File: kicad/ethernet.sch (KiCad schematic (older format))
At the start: 32 parts, among them IC201 TPD4E001QDBV, J201 0821-1X1T-36-F, U201 DP83822

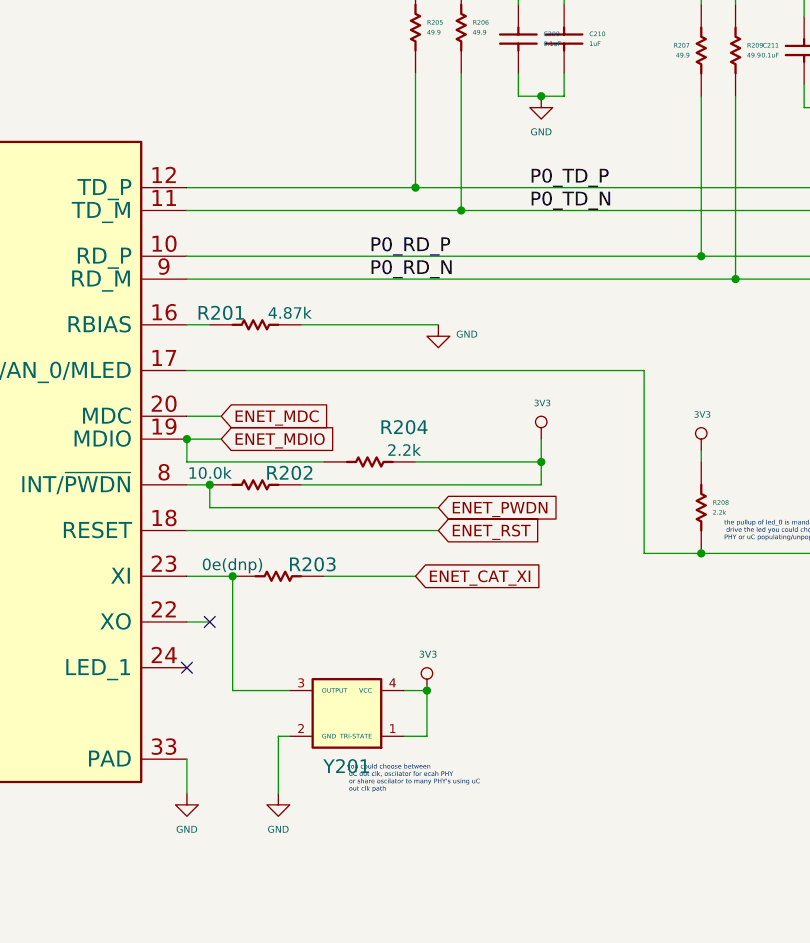
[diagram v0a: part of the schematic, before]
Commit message: keep placing
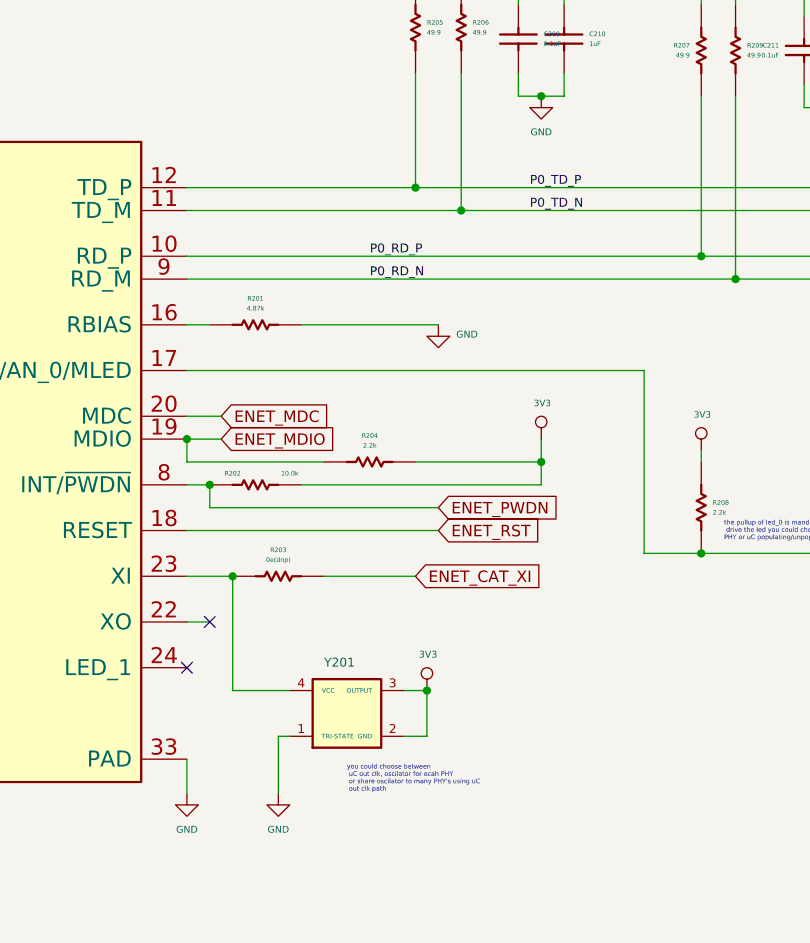
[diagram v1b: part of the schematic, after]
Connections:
- net 3V3: now also R204.2, Y201.2 (GND), Y201.3 (OUTPUT); no longer R204.1, Y201.1 (TRI-STATE), Y201.4 (VCC)
- net ENET_MDIO: now also R204.1; no longer R204.2
- net GND: now also Y201.1 (TRI-STATE); no longer Y201.2 (GND)
- net at R203.1, U201.23 (XI): now also Y201.4 (VCC); no longer Y201.3 (OUTPUT)
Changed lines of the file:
@@
 	1    0    0    -1
 $EndComp
-Text Label 10050 2800 0    60   ~ 0
+Text Label 10050 2800 0    39   ~ 0
 P0_TD_P
-Text Label 10050 2900 0    60   ~ 0
+Text Label 10050 2900 0    39   ~ 0
 P0_TD_N
-Text Label 9350 3100 0    60   ~ 0
+Text Label 9350 3100 0    39   ~ 0
 P0_RD_P
-Text Label 9350 3200 0    60   ~ 0
+Text Label 9350 3200 0    39   ~ 0
 P0_RD_N
 $Comp
@@
 U 1 1 63C6814C
 P 9350 4000
-F 0 "R204" H 9200 3850 60  0000 C CNN
-F 1 "2.2k" H 9200 3950 50  0000 C CNN
-F 2 "Resistor_SMD:R_0603_1608Metric" H 9350 4000 50  0001 C CNN
-F 3 "" H 9350 4000 50  0001 C CNN
+F 0 "R204" H 9350 4115 20  0000 C CNN
+F 1 "2.2k" H 9350 4072 20  0000 C CNN
+F 2 "Resistor_SMD:R_0603_1608Metric" H 8850 3900 60  0001 C CNN
+F 3 "" H 8950 4000 60  0001 C CNN
 F 4 "2.2k" V -150 2900 60  0001 C CNN "ValueDisplayed"
 	1    9350 4000
-	-1   0    0    1
+	1    0    0    -1
 $EndComp
 $Comp
@@
 U 1 1 63C681B2
 P 8850 3400
-F 0 "R201" H 8700 3450 60  0000 C CNN
-F 1 "4.87k" H 9000 3450 50  0000 C CNN
-F 2 "Resistor_SMD:R_0603_1608Metric" H 8850 3400 50  0001 C CNN
-F 3 "" H 8850 3400 50  0001 C CNN
+F 0 "R201" H 8850 3515 20  0000 C CNN
+F 1 "4.87k" H 8850 3472 20  0000 C CNN
+F 2 "Resistor_SMD:R_0603_1608Metric" H 8350 3300 60  0001 C CNN
+F 3 "" H 8450 3400 60  0001 C CNN
 F 4 "4.87k" V -150 2900 60  0001 C CNN "ValueDisplayed"
 	1    8850 3400
@@
 U 1 1 63C681CA
 P 8850 4100
-F 0 "R202" H 9000 4150 60  0000 C CNN
-F 1 "10.0k" H 8650 4150 50  0000 C CNN
-F 2 "Resistor_SMD:R_0603_1608Metric" H 8850 4100 50  0001 C CNN
-F 3 "" H 8850 4100 50  0001 C CNN
+F 0 "R202" H 8750 4150 20  0000 C CNN
+F 1 "10.0k" H 9000 4150 20  0000 C CNN
+F 2 "Resistor_SMD:R_0603_1608Metric" H 8350 4000 60  0001 C CNN
+F 3 "" H 8450 4100 60  0001 C CNN
 F 4 "10.0k" V -150 2900 60  0001 C CNN "ValueDisplayed"
 	1    8850 4100
@@
 U 1 1 63C68282
 P 8950 4500
-F 0 "R203" H 9100 4550 60  0000 C CNN
-F 1 "0e(dnp)" H 8750 4550 50  0000 C CNN
-F 2 "Resistor_SMD:R_0603_1608Metric" H 8950 4500 50  0001 C CNN
-F 3 "" H 8950 4500 50  0001 C CNN
+F 0 "R203" H 8950 4615 20  0000 C CNN
+F 1 "0e(dnp)" H 8950 4572 20  0000 C CNN
+F 2 "Resistor_SMD:R_0603_1608Metric" H 8450 4400 60  0001 C CNN
+F 3 "" H 8550 4500 60  0001 C CNN
 F 4 "10.0k" V -50 3300 60  0001 C CNN "ValueDisplayed"
 	1    8950 4500
@@
 AR Path="/5DC3DC9E/63C6828B" Ref="Y201"  Part="1"
 AR Path="/5DC4A59D/63C6828B" Ref="Y?"  Part="1"
-F 0 "Y201" H 9250 4867 60  0000 C CNN
-F 1 "~" H 9250 5100 50  0001 C CNN
-F 2 "Oscillator:Oscillator_SMD_SeikoEpson_SG210-4Pin_2.5x2.0mm" H 9250 5100 50  0001 C CNN
-F 3 "../doc/datasheets//ECS-2520S.pdf" H 9250 5100 50  0001 C CNN
+F 0 "Y201" H 9150 5300 39  0000 L BNN
+F 1 "~" H 9250 5350 39  0000 C CNN
+F 2 "Oscillator:Oscillator_SMD_SeikoEpson_SG210-4Pin_2.5x2.0mm" H 9300 5050 60  0001 C CNN
+F 3 "../doc/datasheets//ECS-2520S.pdf" H 9150 5650 60  0001 C CNN
 	1    9250 5100
-	-1   0    0    -1
-$EndComp
-$Comp
+	1    0    0    -1
+$EndComp
+$Comp
